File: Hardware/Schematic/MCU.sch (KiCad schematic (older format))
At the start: 12 parts

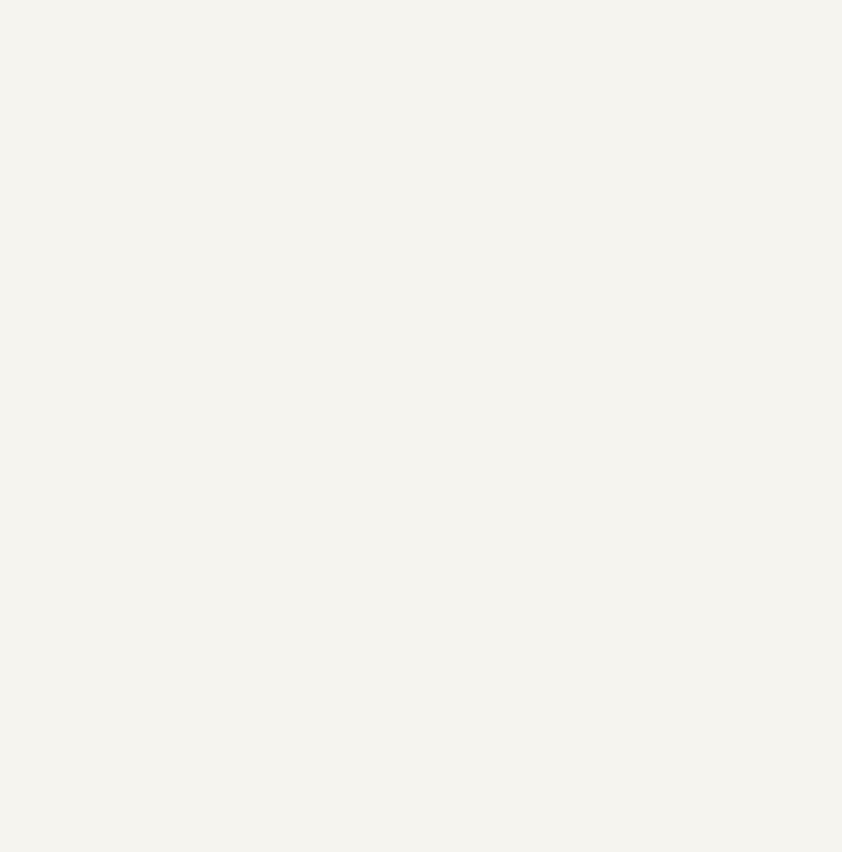
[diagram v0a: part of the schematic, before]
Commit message: Add files via upload
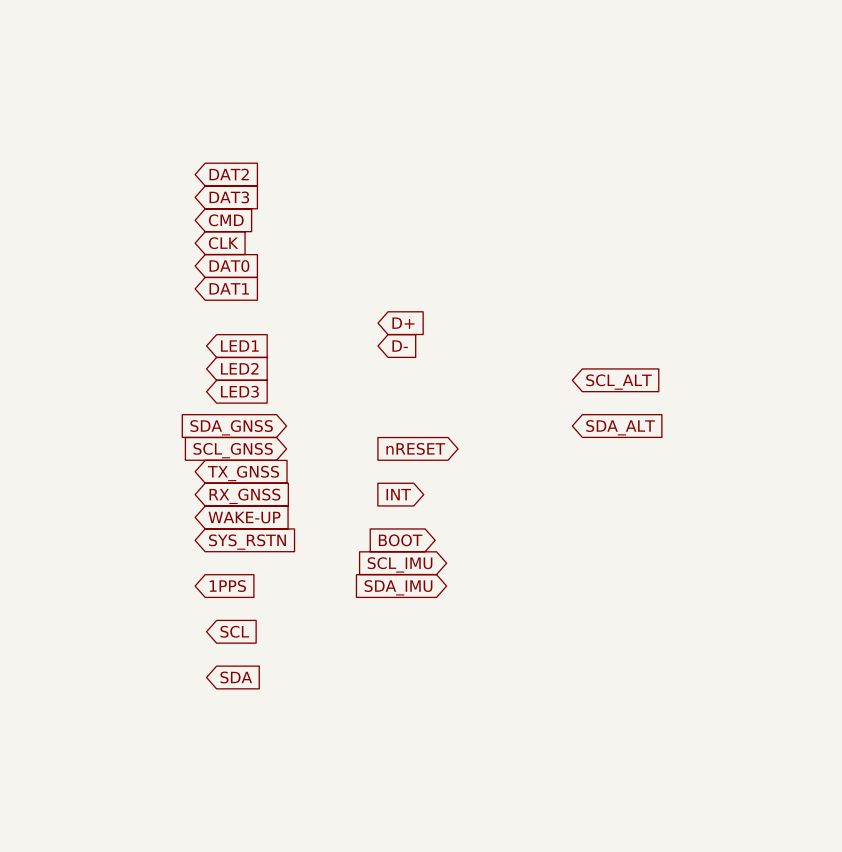
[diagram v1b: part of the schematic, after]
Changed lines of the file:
@@
 $Descr A4 11693 8268
 encoding utf-8
-Sheet 2 4
-Title ""
-Date ""
-Rev ""
-Comp ""
+Sheet 2 5
+Title "ProRTK: All in one Real Time Kinematic device"
+Date "2021-05-12"
+Rev "1"
+Comp "Blackshield Engineering"
 Comment1 ""
 Comment2 ""
@@
 Wire Wire Line
 	2900 3650 2900 3450
+Text GLabel 8950 3550 2    50   Input ~ 0
+D+
+Text GLabel 8950 3650 2    50   Input ~ 0
+D-
+Text GLabel 9800 4000 2    50   Input ~ 0
+SDA_ALT
+Text GLabel 9800 3800 2    50   Input ~ 0
+SCL_ALT
+Text GLabel 9250 4700 0    50   Input ~ 0
+SDA_IMU
+Text GLabel 9250 4600 0    50   Input ~ 0
+SCL_IMU
+Text GLabel 9200 4500 0    50   Input ~ 0
+BOOT
+Text GLabel 9150 4300 0    50   Input ~ 0
+INT
+Text GLabel 9300 4100 0    50   Input ~ 0
+nRESET
+Text GLabel 8200 5100 2    50   Input ~ 0
+SDA
+Text GLabel 8200 4900 2    50   Input ~ 0
+SCL
+Text GLabel 8150 4700 2    50   Input ~ 0
+1PPS
+Text GLabel 8150 4500 2    50   Input ~ 0
+SYS_RSTN
+Text GLabel 8150 4400 2    50   Input ~ 0
+WAKE-UP
+Text GLabel 8150 4300 2    50   Input ~ 0
+RX_GNSS
+Text GLabel 8150 4200 2    50   Input ~ 0
+TX_GNSS
+Text GLabel 8550 4000 0    50   Input ~ 0
+SDA_GNSS
+Text GLabel 8550 4100 0    50   Input ~ 0
+SCL_GNSS
+Text GLabel 8200 3850 2    50   Input ~ 0
+LED3
+Text GLabel 8200 3750 2    50   Input ~ 0
+LED2
+Text GLabel 8200 3650 2    50   Input ~ 0
+LED1
+Text GLabel 8150 3300 2    50   Input ~ 0
+DAT0
+Text GLabel 8150 3400 2    50   Input ~ 0
+DAT1
+Text GLabel 8150 3200 2    50   Input ~ 0
+CLK
+Text GLabel 8150 3100 2    50   Input ~ 0
+CMD
+Text GLabel 8150 2900 2    50   Input ~ 0
+DAT2
+Text GLabel 8150 3000 2    50   Input ~ 0
+DAT3
 $EndSCHEMATC
